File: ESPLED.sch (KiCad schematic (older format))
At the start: 51 parts, among them CON1 BARREL_JACK, J1 USB_B_Micro, J2 LED_CON_RGB, J3 LED_CON_WW, J4 MIC, P1 LED_CON_SCREW, P2 LED_CON_SCREW, P3 LED_CON_SCREW, Q1 IRLZ34N, Q2 IRLZ34N, Q3 IRLZ34N, Q4 IRLZ34N, Q5 IRLZ34N, SW1 Reset, SW2 Program, SW3 Mode, U1 AMS1117-3.3, U2 ESP-07v2, U3 INTERFACE-CH340G, U4 DS18B20, U5 TXS0108EPW, Y1 Crystal

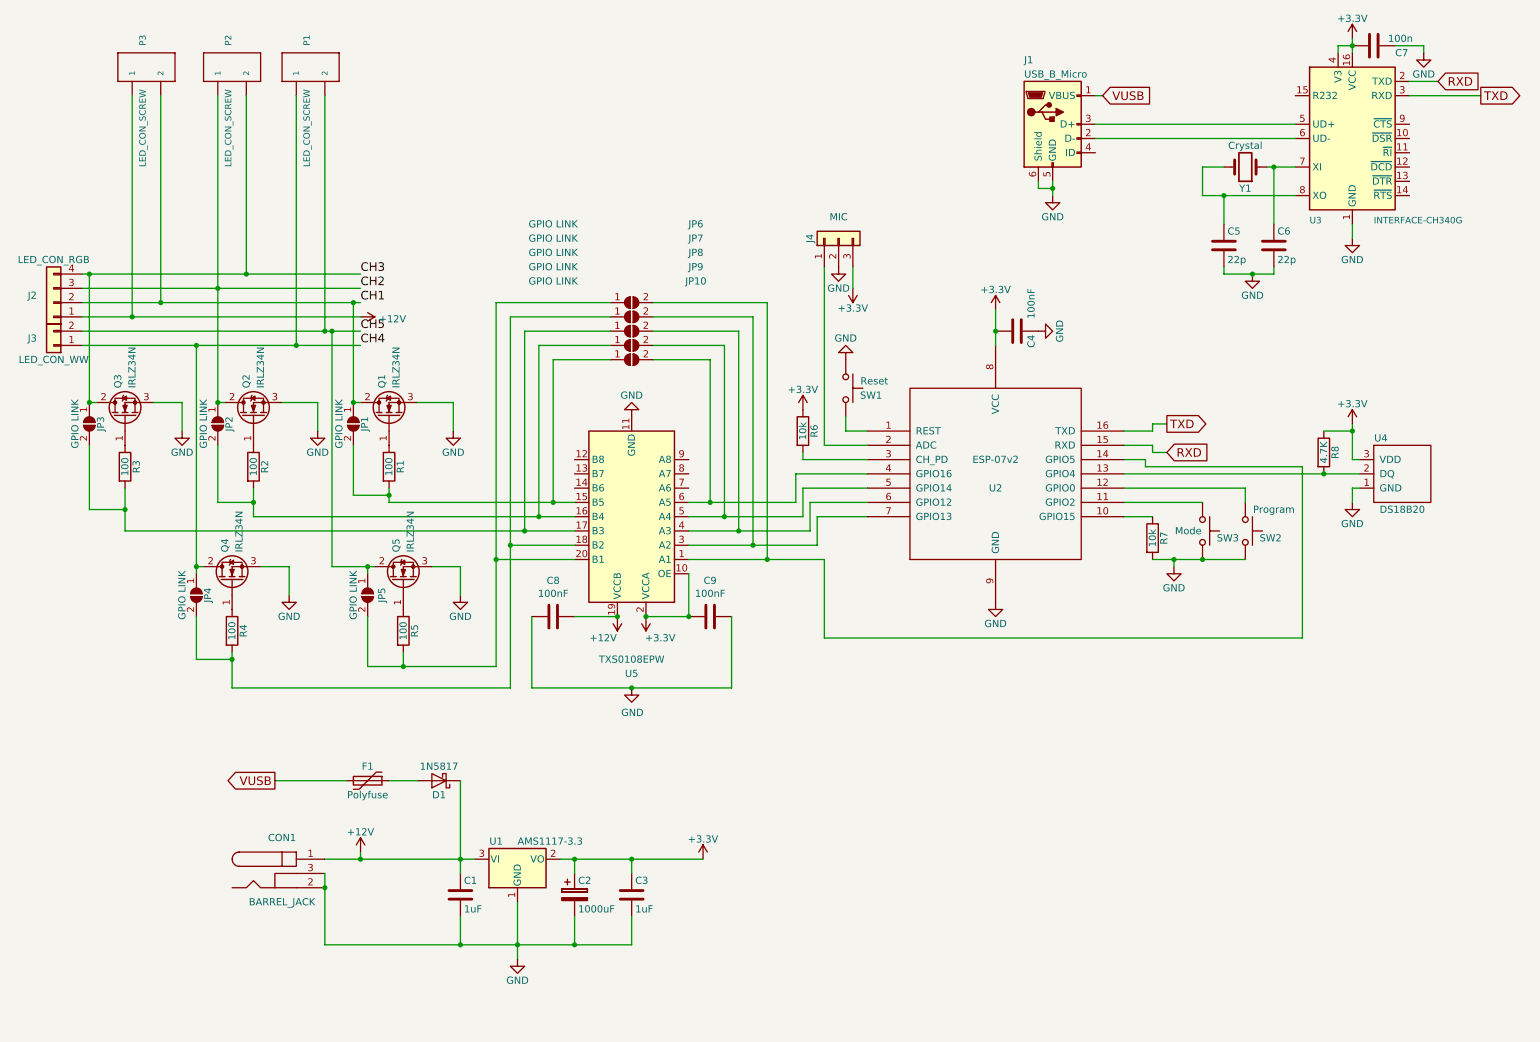
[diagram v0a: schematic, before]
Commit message: Routed
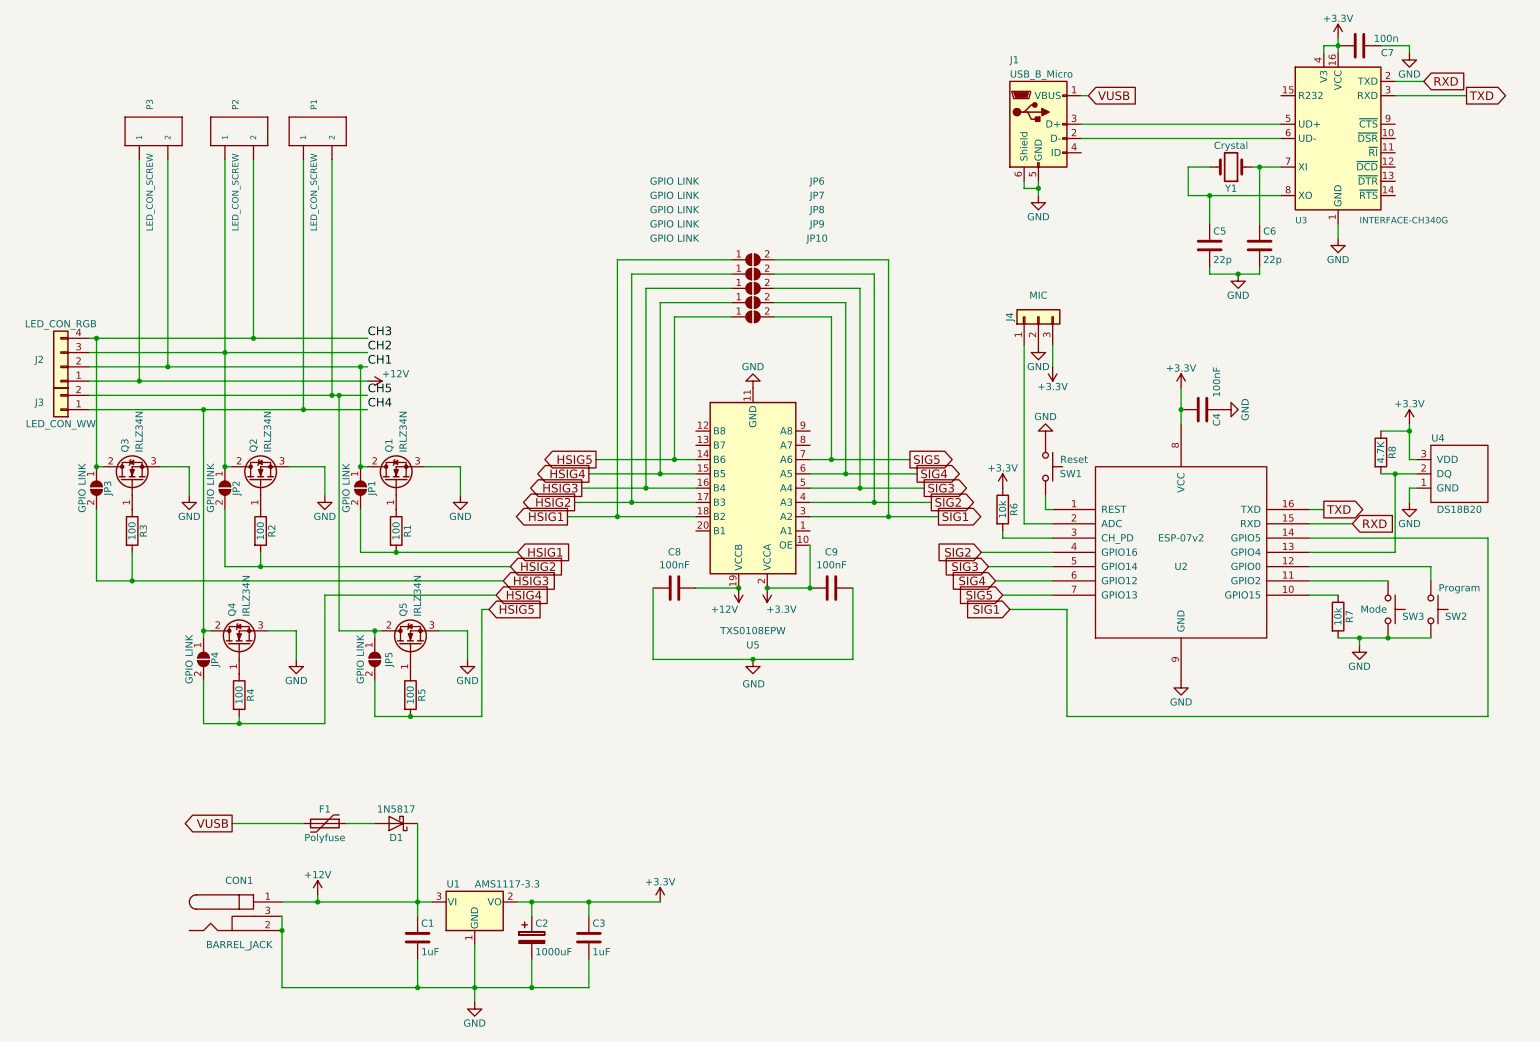
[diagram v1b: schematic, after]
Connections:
- net SIG1: now reaches JP6.2 (B), U2.14 (GPIO5)
- net SIG1: now also U5.3 (A2); no longer U5.1 (A1)
- net SIG3: now reaches U2.5 (GPIO14), U5.5 (A4)
- net SIG3: now also JP8.2 (B); no longer JP9.2 (B)
- net HSIG1: now reaches JP1.2 (B), R1.2
- net HSIG1: now also JP6.1 (A), U5.18 (B2); no longer JP10.1 (A), U5.15 (B5)
- net HSIG2: now reaches JP2.2 (B), R2.2
- net HSIG2: now also JP7.1 (A), U5.17 (B3); no longer JP9.1 (A), U5.16 (B4)
- net HSIG3: now reaches JP3.2 (B), JP8.1 (A), R3.2
- net HSIG3: now also U5.16 (B4); no longer U5.17 (B3)
- net HSIG4: now reaches JP4.2 (B), R4.2
- net HSIG4: now also JP9.1 (A), U5.15 (B5); no longer JP7.1 (A), U5.18 (B2)
- net HSIG5: now reaches JP5.2 (B), R5.2
- net HSIG5: now also JP10.1 (A), U5.14 (B6); no longer JP6.1 (A), U5.20 (B1)
- net SIG5: now reaches U5.7 (A6)
- net SIG5: now also JP10.2 (B), U2.7 (GPIO13)
- new net SIG2: JP7.2 (B), U2.4 (GPIO16), U5.4 (A3)
- new net SIG4: JP9.2 (B), U2.6 (GPIO12), U5.6 (A5)
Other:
- moved on the sheet: C1, C2, C3, C4, C5, C6, C7, C8, C9, CON1, D1, F1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
